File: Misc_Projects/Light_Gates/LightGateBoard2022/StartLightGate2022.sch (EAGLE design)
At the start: 6 parts

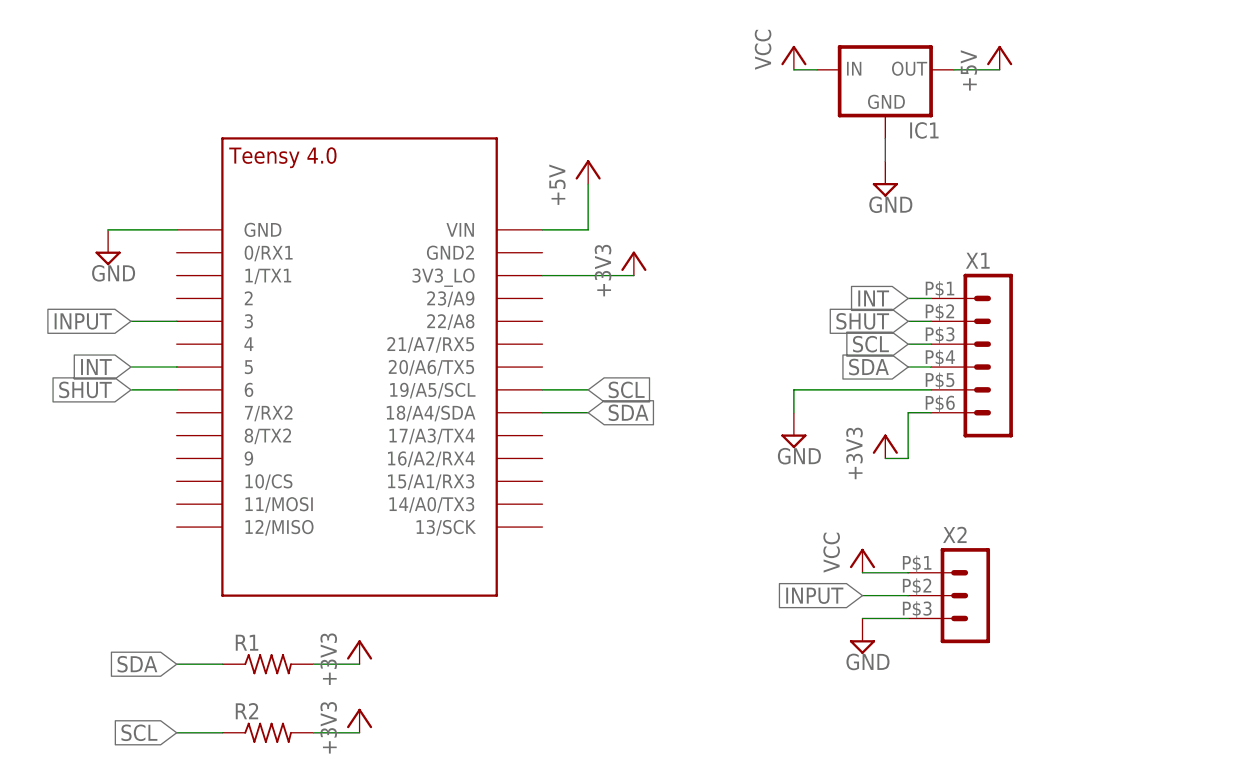
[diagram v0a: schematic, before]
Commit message: Light Gate Updates
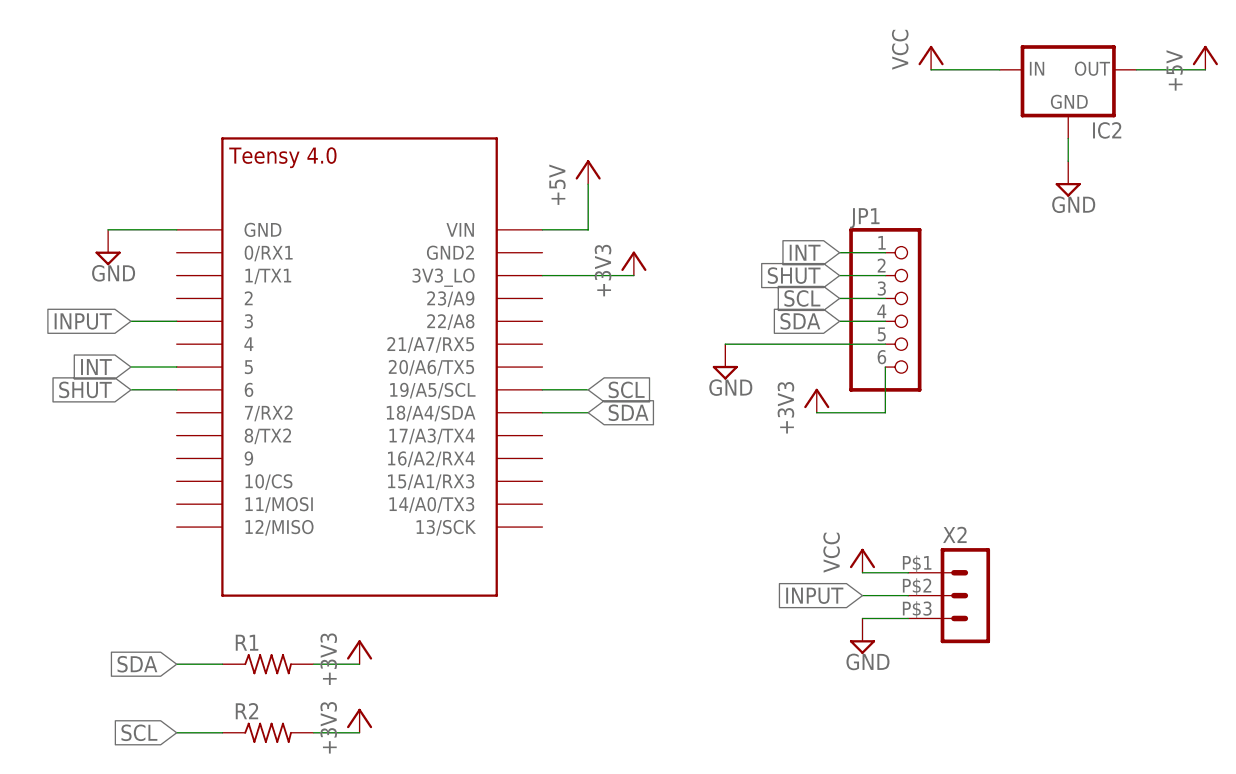
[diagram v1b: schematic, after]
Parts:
- removed IC1: (no value), GTOR - Active Components:REG_5V_L7805_VERT
- removed X1: (no value), GTOR - Microfit Connector:HEADER_POS6_43045-0600
- added IC2: (no value), GTOR - Active Components:REG_5V_L7805_HOR
- added JP1: (no value), GTOR - Connectors:PINHD-1X6
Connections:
- net +3V3: now also JP1.6; no longer X1.6
- net +5V: now also IC2.OUT; no longer IC1.OUT
- net GND: now also IC2.GND, JP1.5; no longer IC1.GND, X1.5
- net INT: now also JP1.1; no longer X1.1
- net SCL: now also JP1.3; no longer X1.3
- net SDA: now also JP1.4; no longer X1.4
- net SHUT: now also JP1.2; no longer X1.2
- net VCC: now also IC2.IN; no longer IC1.IN
